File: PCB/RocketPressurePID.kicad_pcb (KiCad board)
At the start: 2 copper layers, 58 x 47 mm, 48 parts, among them J1 TYPE-C 16PIN 2MD(073), J2 2x14 1.27mm SMD, J6 S5B-PH-SM4-TB(LF)(SN), Q4 IRLML2502TRPBF, SW1 TS-1002S-08026C, SW2 TS-1002S-08026C, U2 HS HS13L03W2C01, U3 AMS1117-3.3, U4 M24C02-FMN, U5 STM32G030C8Tx, Y2 8 MHz

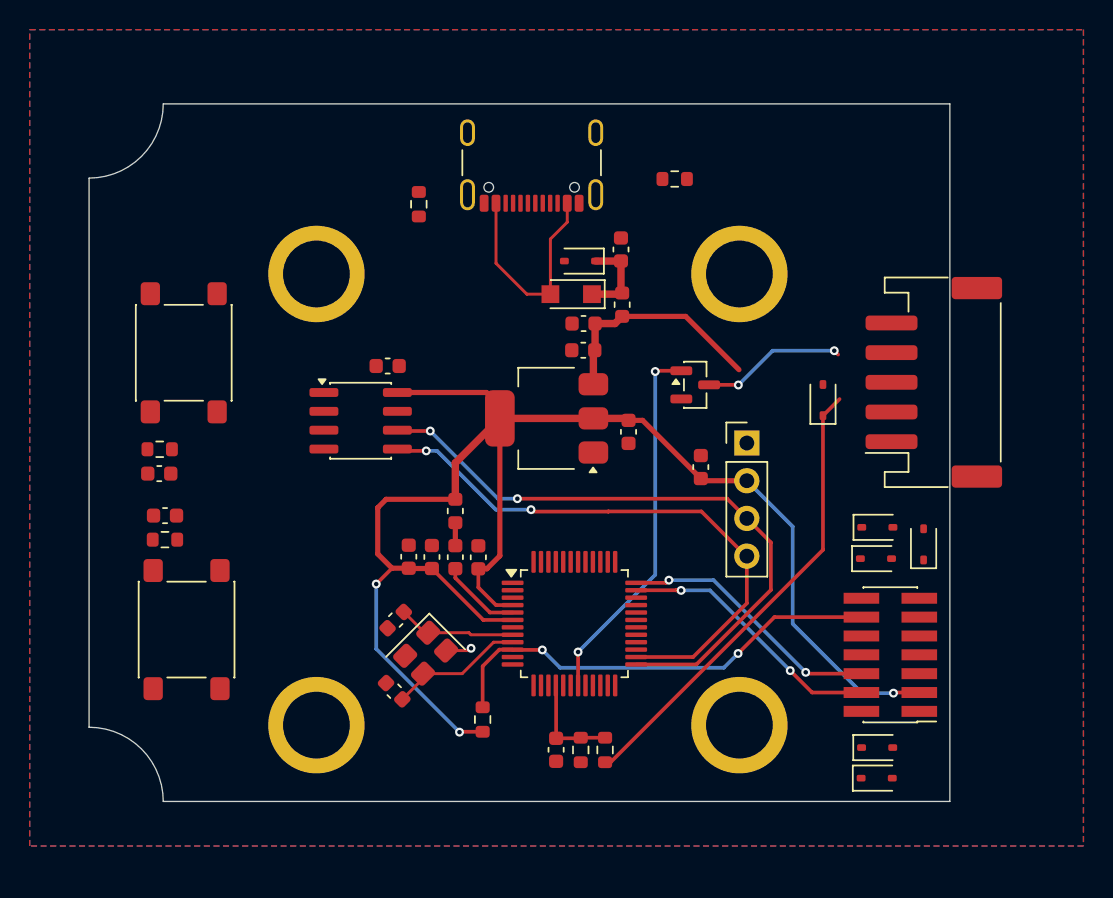
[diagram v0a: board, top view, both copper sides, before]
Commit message: WIP
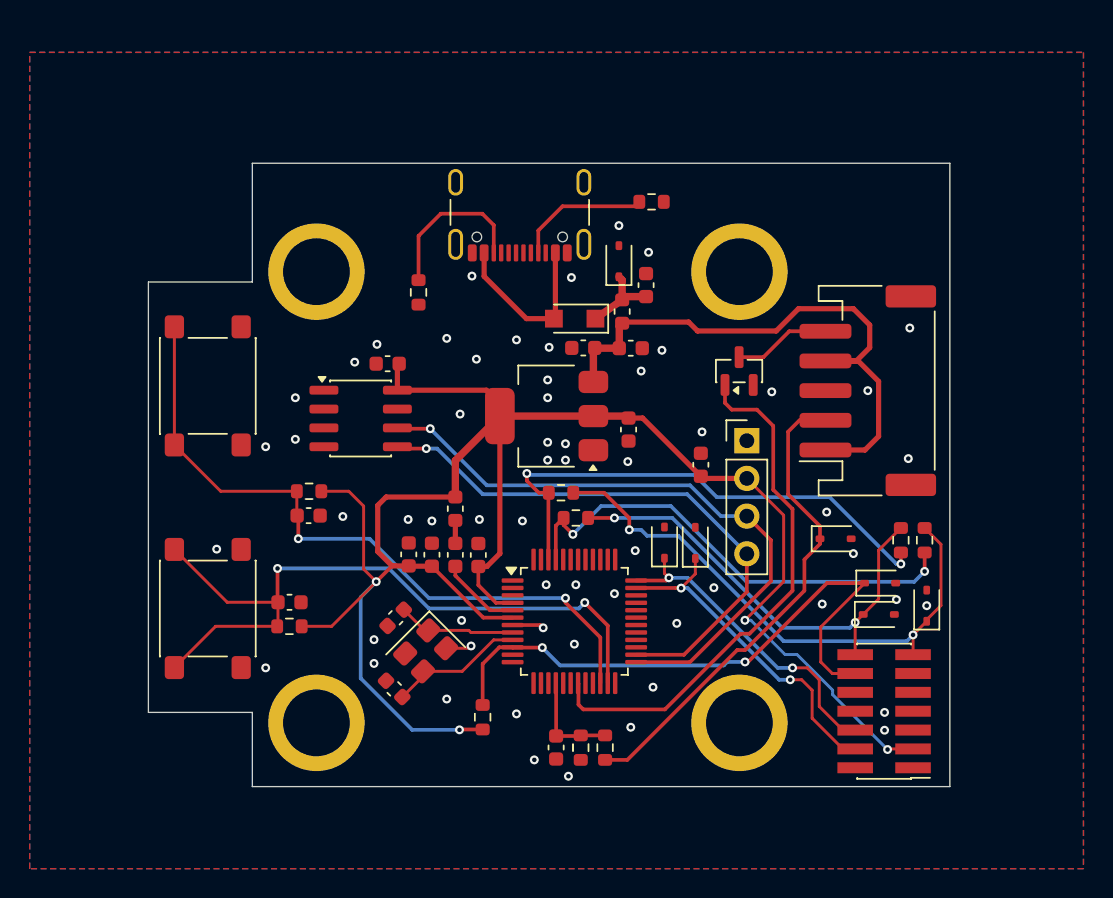
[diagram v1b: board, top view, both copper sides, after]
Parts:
- added R10: 0R, Resistor_SMD:R_0603_1608Metric, F.Cu at (130.8, 85.2)
- added R11: 0R, Resistor_SMD:R_0603_1608Metric, F.Cu at (155.3, 88.4)
- added R12: 0R, Resistor_SMD:R_0603_1608Metric, F.Cu at (153.7, 88.4)
- added R9: 0R, Resistor_SMD:R_0603_1608Metric, F.Cu at (131.8, 86.9)
- moved D15 21.4 mm to (137.8, 88.6), turned to 90 degrees
- moved D16 18.4 mm to (139.8, 88.6), turned to 90 degrees
- moved C15 10.5 mm to (113.8, 86.7)
- moved R3 10.5 mm to (113.8, 85.1)
- moved R4 10.2 mm to (112.5, 94.2)
- moved C16 10.2 mm to (112.5, 92.6)
- moved D20 9.38 mm to (149.3, 88.3), turned to 0 degrees
- moved R7 5.94 mm to (121.2, 71.7)
- moved J6 4.49 mm to (151.5, 78.3)
- moved D19 4.14 mm to (155.4, 92.8)
- moved J2 3.82 mm to (152.6, 99.9)
- moved D14 3.76 mm to (152.3, 91.3)
- moved D18 3.76 mm to (152.2, 93.4)
- moved C1 3.59 mm to (135.5, 75.5), turned to 0 degrees
- moved J1 3.44 mm to (128.0, 65.4)
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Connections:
- D18 pad 1: /MCU_DBG_TX -> Net-(D18-A1)
- D19 pad 1: /MCU_DBG_RX -> Net-(D19-A1)
- J2 pad 13: /MCU_DBG_RX -> Net-(D19-A1)
- J2 pad 14: /MCU_DBG_TX -> Net-(D18-A1)
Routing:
- net /~{SW_DOWN}: track 0.00 -> 48.5 mm, vias 0 -> 2
- net /~{SW_UP}: track 0.00 -> 47.1 mm, vias 0 -> 2
- net Net-(D19-A1): track 0.00 -> 37.4 mm, vias 0 -> 2
- net /MCU_DBG_RX: track 0.00 -> 35.3 mm, vias 0 -> 2
- net /MCU_DBG_TX: track 0.00 -> 32.5 mm, vias 0 -> 2
- net Net-(D18-A1): track 0.00 -> 31.0 mm, vias 0 -> 2
- net +5V: track 15.5 -> 40.5 mm
- net +3.3V: track 106.0 -> 130.9 mm, vias 3 -> 4
- net /SSR_EN: track 25.1 -> 36.1 mm, vias 2 -> 0
- net Net-(J1-CC2): track 0.00 -> 10.9 mm
- net /~{MCU_RESET}: track 30.7 -> 40.9 mm
- net Net-(J1-CC1): track 0.00 -> 9.11 mm
- net /SWDIO: track 18.0 -> 22.7 mm
- net /SWCLK: track 17.9 -> 21.6 mm
- net Net-(D1-A): track 15.2 -> 11.9 mm
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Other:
- board size 58 x 47 mm -> 54 x 42 mm
- board text added: "MYLA'S CIRCUIT BOARD"
- board text added: "PID Controller v1.0"
